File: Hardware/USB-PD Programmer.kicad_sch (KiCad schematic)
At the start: 29 parts, among them J1 Conn_01x07_Male, J2 Conn_01x04_Male, J3 Conn_01x02_Male, J4 Conn_01x02_Male, J5 Conn_01x02_Male, J6 Conn_01x02_Male, J7 Conn_01x08_Male, J9 QWIIC_Stackable, SW1 SW_Push, U1 R1501J033B-T1-JE, U2 CH340G/C, Y1 12M

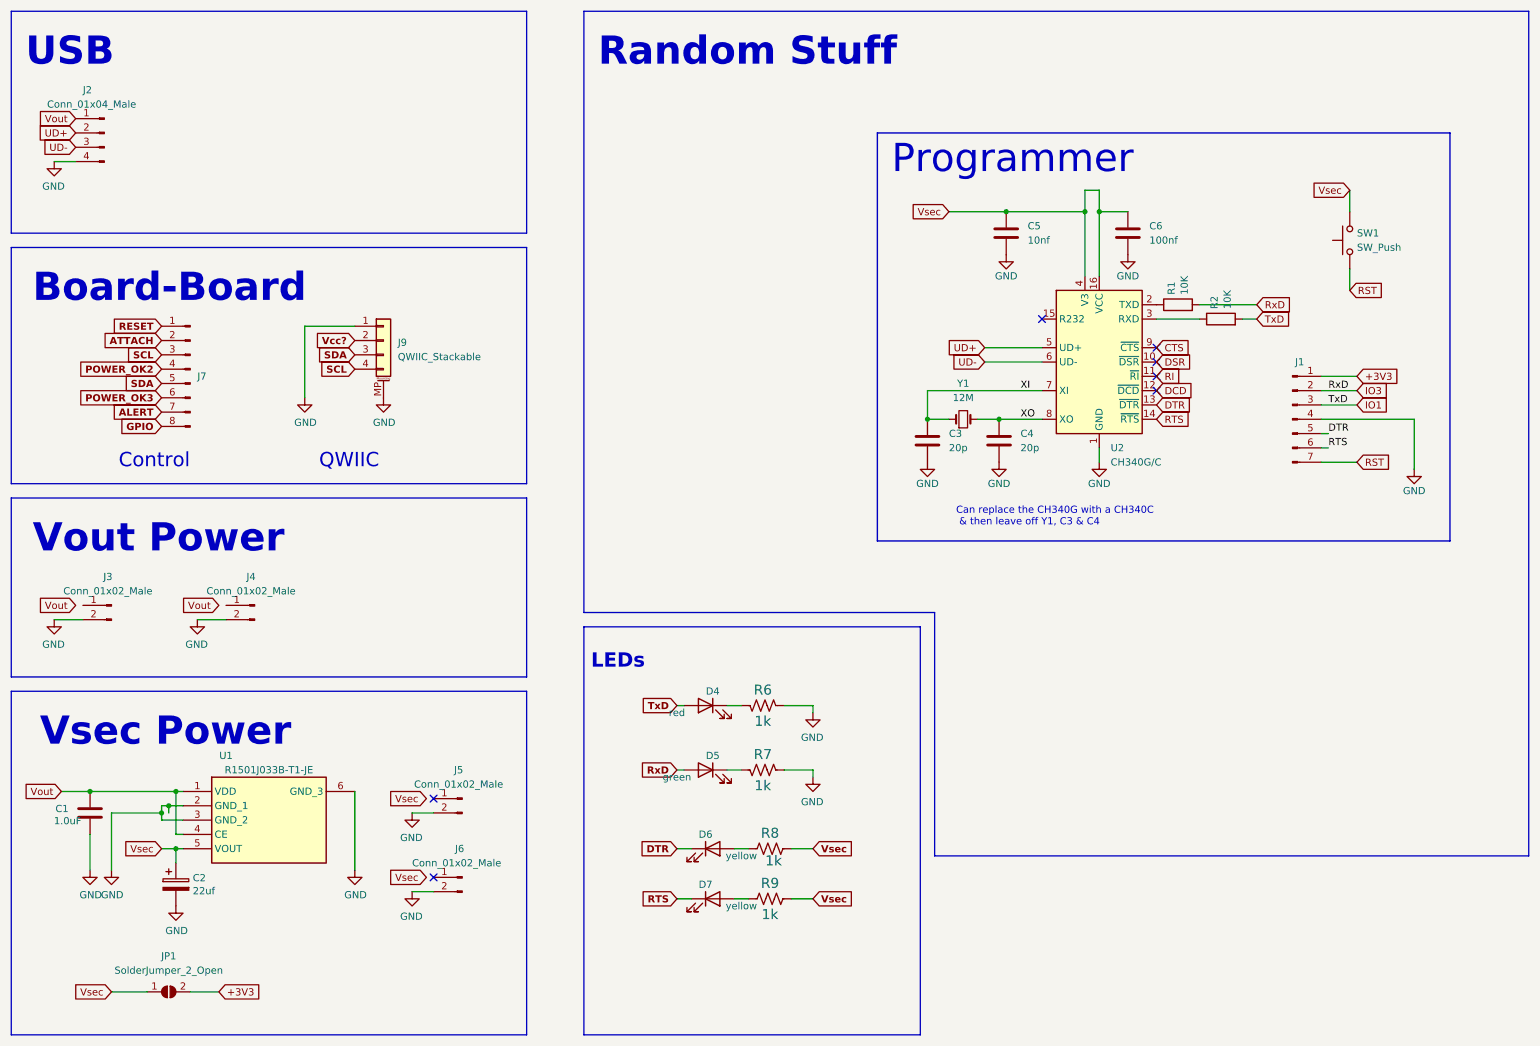
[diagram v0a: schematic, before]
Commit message: Rabbit OCD attack...
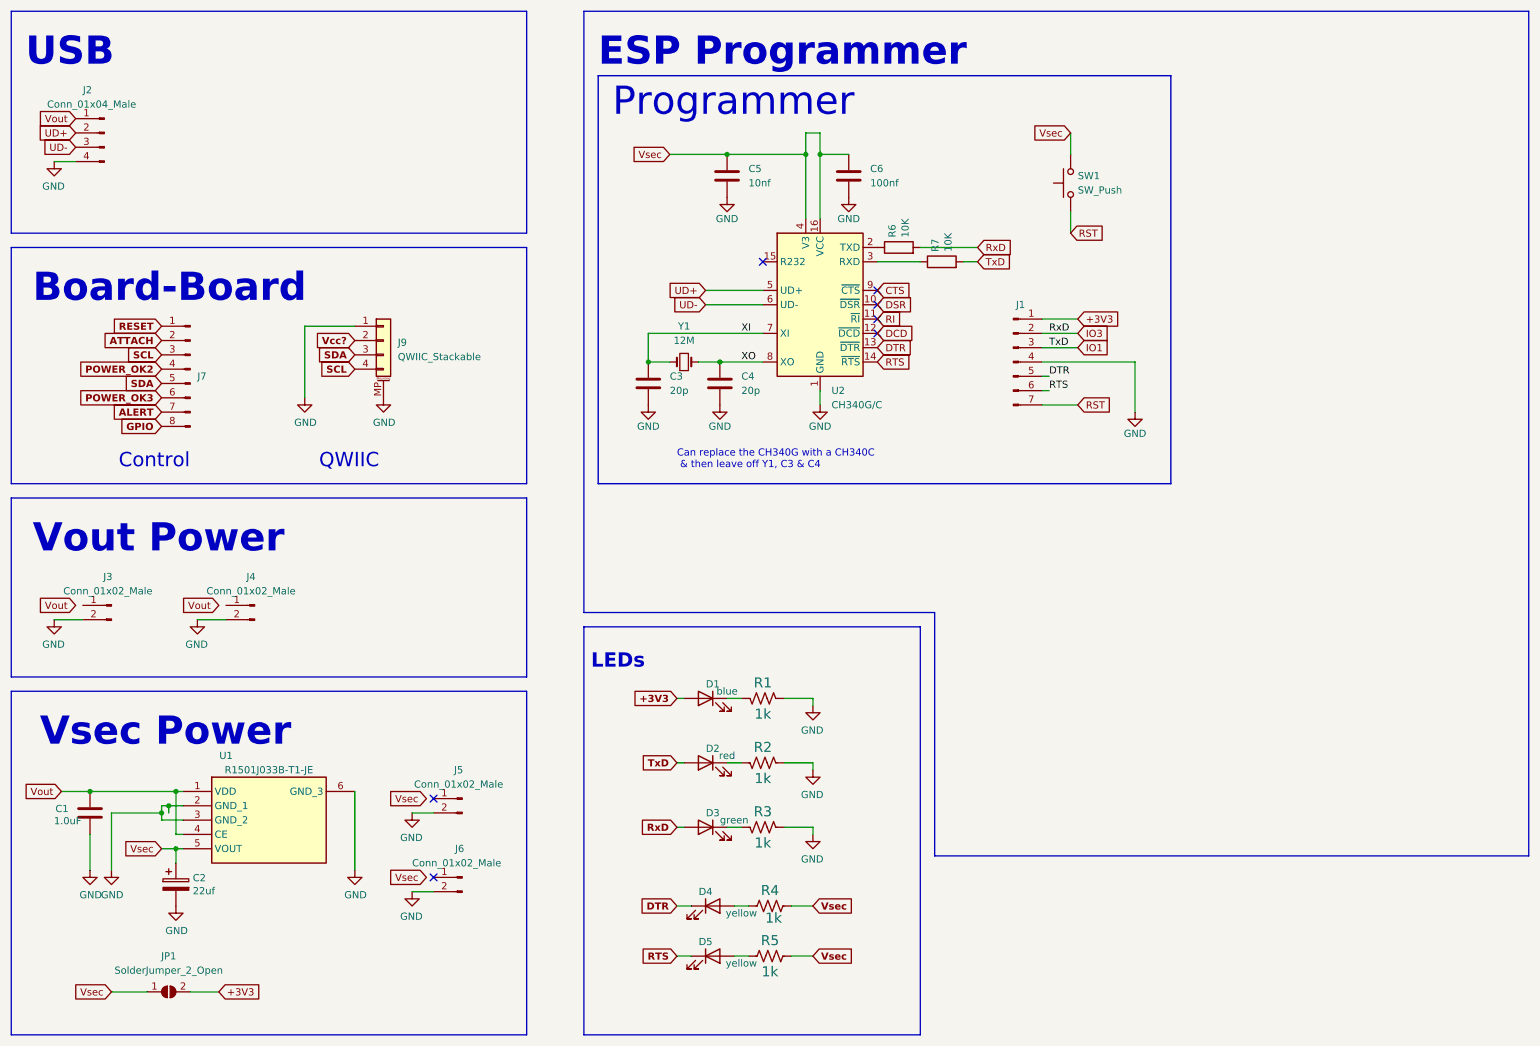
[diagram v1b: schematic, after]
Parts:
- added D1: blue, LED_SMD:LED_0603_1608Metric, symbol Device:LED
- added R1: 1k, Resistor_SMD:R_0603_1608Metric, symbol Device:R_US
- renumbered D4 to D2, D5 to D3, D6 to D4, D7 to D5, R6 to R2, R7 to R3, R8 to R4, R9 to R5, R1 to R6, R2 to R7
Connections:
- net +3V3: now also D1.2 (A)
- net GND: now also R1.1
- new net: D1.1 (K), R1.2
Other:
- note added: "ESP Programmer"
- note removed: "Random Stuff"
- moved on the sheet: C3, C4, C5, C6, D2, D3, D4, D5, J1, R2, R3, R4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
